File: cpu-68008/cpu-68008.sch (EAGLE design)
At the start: 54 parts, among them IC1 68008, IC11 NE555, IC2 AS6C4008, IC3 39SF010, IC4 DS1244Y, IC5 XR68C681, Q1 8MHz, Q2 3.6864MHz

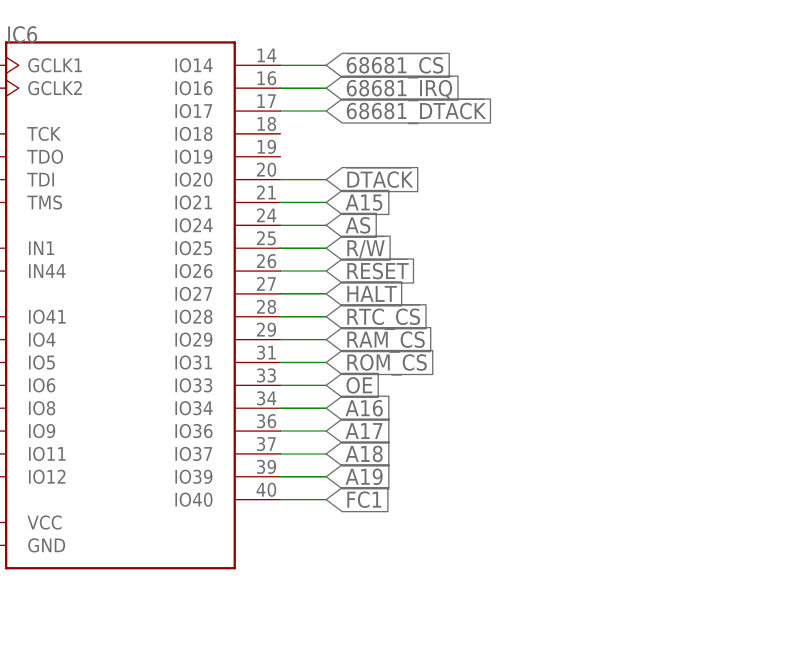
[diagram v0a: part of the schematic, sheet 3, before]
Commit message: finished routing CPLD
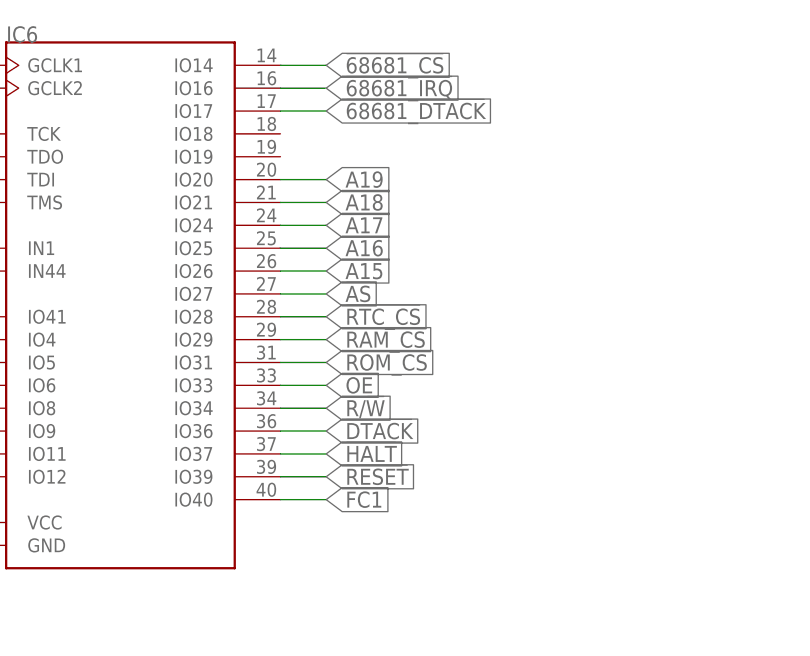
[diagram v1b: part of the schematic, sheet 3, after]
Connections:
- net !AS: now also IC6.IO27; no longer IC6.IO24
- net !DTACK: now also IC6.IO36; no longer IC6.IO20
- net !HALT: now also IC6.IO37; no longer IC6.IO27
- net !RESET: now also IC6.IO39; no longer IC6.IO26
- net A15: now also IC6.IO26; no longer IC6.IO21
- net A16: now also IC6.IO25; no longer IC6.IO34
- net A17: now also IC6.IO24; no longer IC6.IO36
- net A18: now also IC6.IO21; no longer IC6.IO37
- net A19: now also IC6.IO20; no longer IC6.IO39
- net R/!W!: now also IC6.IO34; no longer IC6.IO25
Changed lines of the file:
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@@
 </segment>
 </net>
-<net name="A19" class="0">
+<net name="A17" class="0">
 <segment>
-<pinref part="IC6" gate="G$1" pin="IO39"/>
-<wire x1="83.82" y1="127" x2="88.9" y2="127" width="0.1524" layer="91"/>
-<label x="88.9" y="127" size="1.778" layer="95" xref="yes"/>
+<pinref part="IC6" gate="G$1" pin="IO24"/>
+<wire x1="83.82" y1="154.94" x2="88.9" y2="154.94" width="0.1524" layer="91"/>
+<label x="88.9" y="154.94" size="1.778" layer="95" xref="yes"/>
 </segment>
 </net>
-<net name="A18" class="0">
+<net name="!HALT" class="0">
 <segment>
 <pinref part="IC6" gate="G$1" pin="IO37"/>
@@
 </segment>
 </net>
-<net name="A17" class="0">
+<net name="A15" class="0">
 <segment>
-<pinref part="IC6" gate="G$1" pin="IO36"/>
-<wire x1="83.82" y1="132.08" x2="88.9" y2="132.08" width="0.1524" layer="91"/>
-<label x="88.9" y="132.08" size="1.778" layer="95" xref="yes"/>
+<pinref part="IC6" gate="G$1" pin="IO26"/>
+<wire x1="83.82" y1="149.86" x2="88.9" y2="149.86" width="0.1524" layer="91"/>
+<label x="88.9" y="149.86" size="1.778" layer="95" xref="yes"/>
 </segment>
 </net>
-<net name="A16" class="0">
-<segment>
-<pinref part="IC6" gate="G$1" pin="IO34"/>
-<wire x1="83.82" y1="134.62" x2="88.9" y2="134.62" width="0.1524" layer="91"/>
-<label x="88.9" y="134.62" size="1.778" layer="95" xref="yes"/>
-</segment>
-</net>
-<net name="!HALT" class="0">
+<net name="!AS" class="0">
 <segment>
 <pinref part="IC6" gate="G$1" pin="IO27"/>
@@
 </segment>
 </net>
-<net name="!DTACK" class="0">
-<segment>
-<pinref part="IC6" gate="G$1" pin="IO20"/>
-<wire x1="83.82" y1="160.02" x2="88.9" y2="160.02" width="0.1524" layer="91"/>
-<label x="88.9" y="160.02" size="1.778" layer="95" xref="yes"/>
-</segment>
-</net>
-<net name="A15" class="0">
-<segment>
-<pinref part="IC6" gate="G$1" pin="IO21"/>
-<wire x1="83.82" y1="157.48" x2="88.9" y2="157.48" width="0.1524" layer="91"/>
-<label x="88.9" y="157.48" size="1.778" layer="95" xref="yes"/>
-</segment>
-</net>
-<net name="!AS" class="0">
-<segment>
-<pinref part="IC6" gate="G$1" pin="IO24"/>
-<wire x1="83.82" y1="154.94" x2="88.9" y2="154.94" width="0.1524" layer="91"/>
-<label x="88.9" y="154.94" size="1.778" layer="95" xref="yes"/>
-</segment>
-</net>
 <net name="R/!W!" class="0">
 <segment>
-<pinref part="IC6" gate="G$1" pin="IO25"/>
-<wire x1="83.82" y1="152.4" x2="88.9" y2="152.4" width="0.1524" layer="91"/>
-<label x="88.9" y="152.4" size="1.778" layer="95" xref="yes"/>
-</segment>
-</net>
-<net name="!RESET" class="0">
-<segment>
-<pinref part="IC6" gate="G$1" pin="IO26"/>
-<wire x1="83.82" y1="149.86" x2="88.9" y2="149.86" width="0.1524" layer="91"/>
-<label x="88.9" y="149.86" size="1.778" layer="95" xref="yes"/>
+<pinref part="IC6" gate="G$1" pin="IO34"/>
+<wire x1="83.82" y1="134.62" x2="88.9" y2="134.62" width="0.1524" layer="91"/>
+<label x="88.9" y="134.62" size="1.778" layer="95" xref="yes"/>
 </segment>
 </net>
@@
 </segment>
 </net>
+<net name="!RESET" class="0">
+<segment>
+<pinref part="IC6" gate="G$1" pin="IO39"/>
+<wire x1="83.82" y1="127" x2="88.9" y2="127" width="0.1524" layer="91"/>
+<label x="88.9" y="127" size="1.778" layer="95" xref="yes"/>
+</segment>
+</net>
+<net name="!DTACK" class="0">
+<segment>
+<pinref part="IC6" gate="G$1" pin="IO36"/>
+<wire x1="83.82" y1="132.08" x2="88.9" y2="132.08" width="0.1524" layer="91"/>
+<label x="88.9" y="132.08" size="1.778" layer="95" xref="yes"/>
+</segment>
+</net>
+<net name="A16" class="0">
+<segment>
+<pinref part="IC6" gate="G$1" pin="IO25"/>
+<wire x1="83.82" y1="152.4" x2="88.9" y2="152.4" width="0.1524" layer="91"/>
+<label x="88.9" y="152.4" size="1.778" layer="95" xref="yes"/>
+</segment>
+</net>
+<net name="A18" class="0">
+<segment>
+<pinref part="IC6" gate="G$1" pin="IO21"/>
+<wire x1="83.82" y1="157.48" x2="88.9" y2="157.48" width="0.1524" layer="91"/>
+<label x="88.9" y="157.48" size="1.778" layer="95" xref="yes"/>
+</segment>
+</net>
+<net name="A19" class="0">
+<segment>
+<pinref part="IC6" gate="G$1" pin="IO20"/>
+<wire x1="83.82" y1="160.02" x2="88.9" y2="160.02" width="0.1524" layer="91"/>
+<label x="88.9" y="160.02" size="1.778" layer="95" xref="yes"/>
+</segment>
+</net>
